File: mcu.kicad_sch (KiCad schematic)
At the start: 47 parts, among them J1 USB_C_Receptacle_USB2.0_16P, J4 Conn_01x03_Pin, J5 Conn_01x03_Pin, J6 Conn_02x04_Odd_Even, J7 AudioJack2_Ground_Switch, SW4 RotaryEncoder_Switch, SW5 RESET, SW6 BOOTSEL, U1 RP2040, U5 W25Q64JVSSIQ, U6 ADS1015IDGS, Y1 XYDBPCNANF-12MHZ

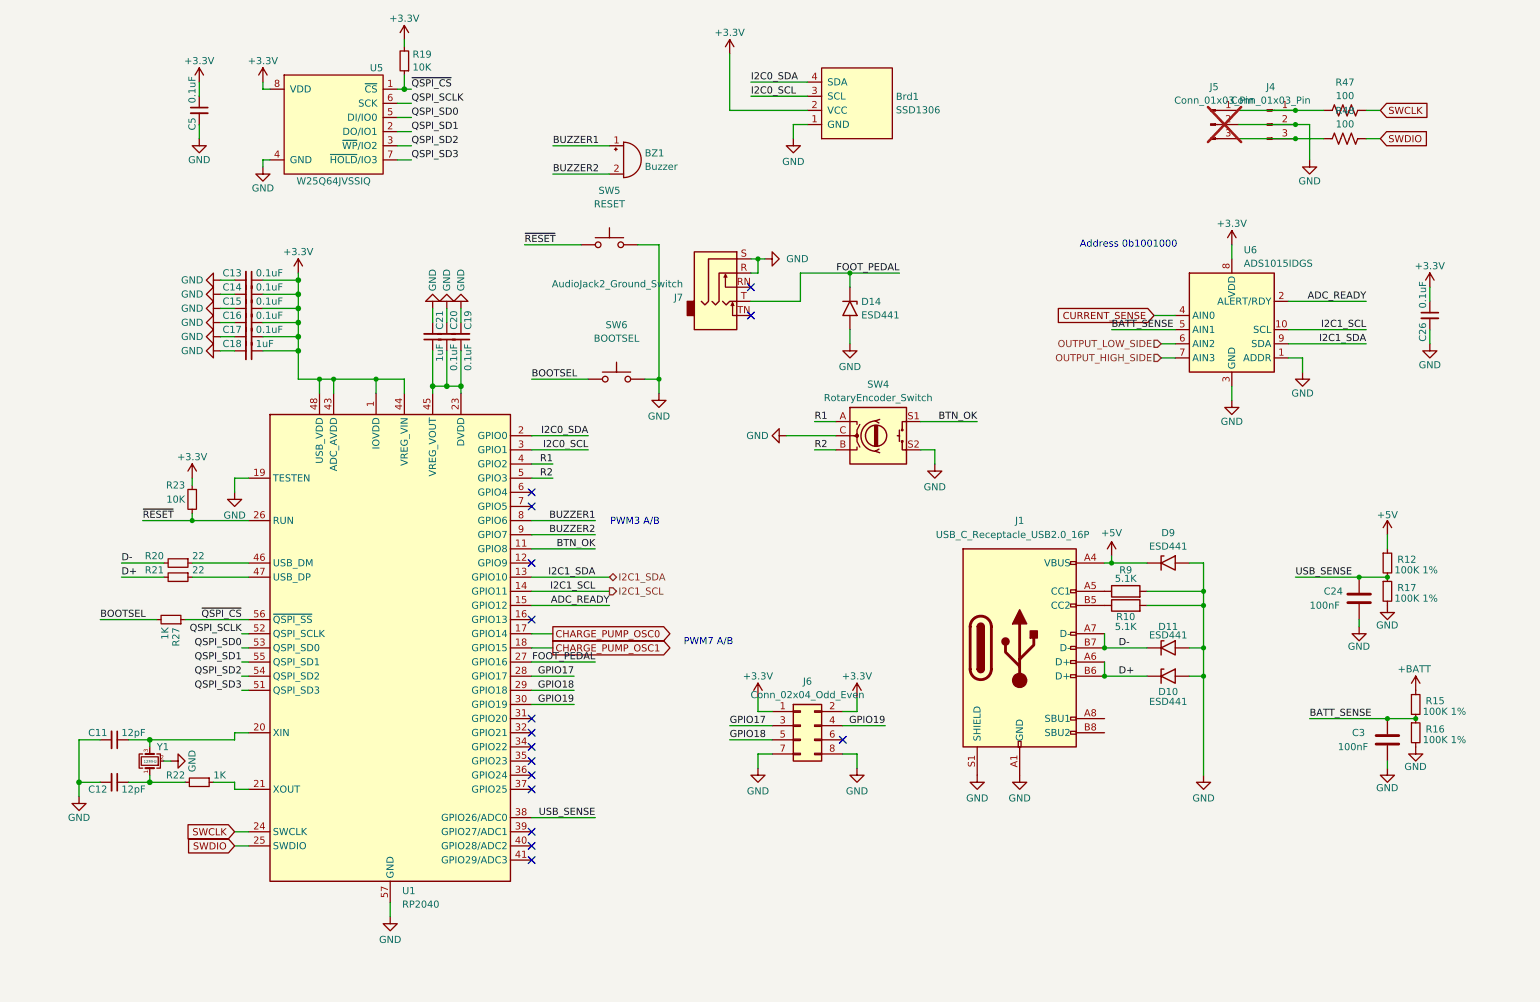
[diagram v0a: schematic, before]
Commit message: stm32g0
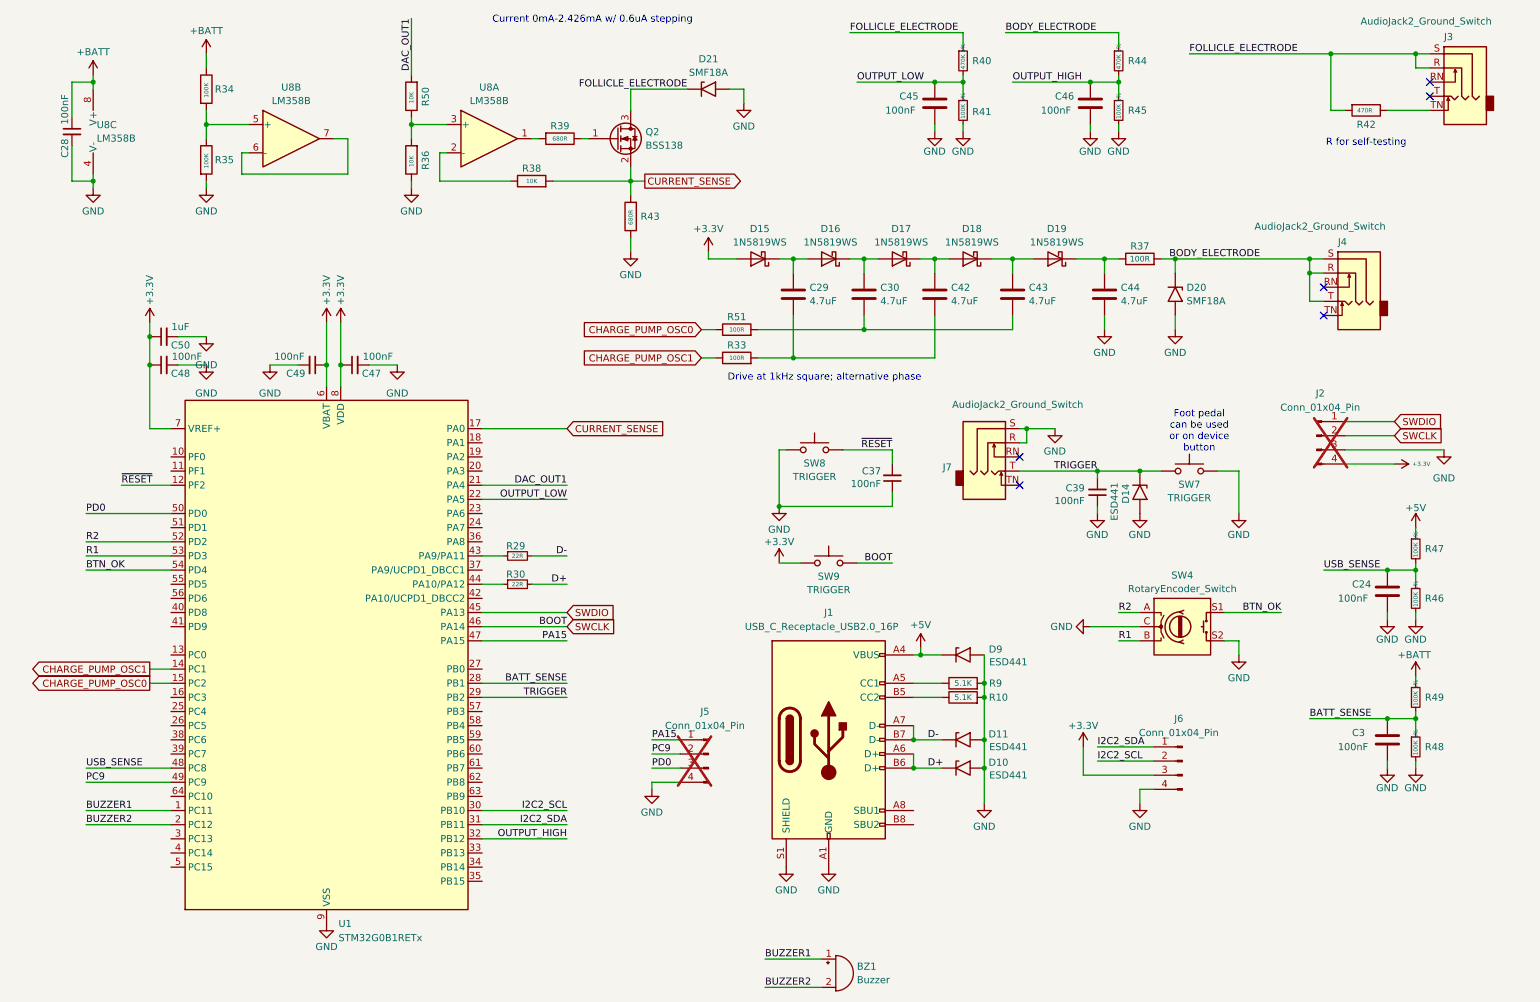
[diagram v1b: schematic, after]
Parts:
- removed Brd1: SSD1306, SSD1306:128x64OLED, symbol SSD1306-128x64_OLED:SSD1306
- removed C11, C12: 12pF, Capacitor_SMD:C_0603_1608Metric, symbol Device:C_Small
- removed C13, C14, C15, C16, C17, C19, C20, C26, C5: 0.1uF, Capacitor_SMD:C_0603_1608Metric, symbol Device:C_Small
- removed C18, C21: 1uF, Capacitor_SMD:C_0603_1608Metric, symbol Device:C_Small
- removed J4: Conn_01x03_Pin, Connector_JST:JST_SH_SM03B-SRSS-TB_1x03-1MP_P1.00mm_Horizontal, symbol Connector:Conn_01x03_Pin
- removed J5: Conn_01x03_Pin, Connector_PinHeader_2.54mm:PinHeader_1x03_P2.54mm_Vertical, symbol Connector:Conn_01x03_Pin
- removed J6: Conn_02x04_Odd_Even, Connector_PinHeader_2.54mm:PinHeader_2x04_P2.54mm_Vertical, symbol Connector_Generic:Conn_02x04_Odd_Even
- removed R12, R15, R16, R17: 100K 1%, Resistor_SMD:R_0603_1608Metric, symbol Device:R_Small
- removed R19, R23: 10K, Resistor_SMD:R_0603_1608Metric, symbol Device:R_Small
- removed R20, R21: 22, Resistor_SMD:R_0603_1608Metric, symbol Device:R_Small
- removed R22, R27: 1K, Resistor_SMD:R_0603_1608Metric, symbol Device:R_Small
- removed R47, R48: 100, Resistor_SMD:R_0603_1608Metric, symbol Device:R_US
- removed SW5: RESET, Button_Switch_SMD:SW_Push_1P1T_NO_E-Switch_TL3301NxxxxxG, symbol Switch:SW_Push
- removed SW6: BOOTSEL, Button_Switch_SMD:SW_Push_1P1T_NO_E-Switch_TL3301NxxxxxG, symbol Switch:SW_Push
- removed U1: RP2040, Package_DFN_QFN:QFN-56-1EP_7x7mm_P0.4mm_EP3.2x3.2mm, symbol MCU_RaspberryPi:RP2040
- removed U5: W25Q64JVSSIQ, Package_SO:SOIC-8_5.3x5.3mm_P1.27mm, symbol Memory_Flash_Extra:GD25Q32C
- removed U6: ADS1015IDGS, Package_SO:TSSOP-10_3x3mm_P0.5mm, symbol Analog_ADC:ADS1015IDGS
- removed Y1: XYDBPCNANF-12MHZ, Crystal:Crystal_SMD_3225-4Pin_3.2x2.5mm, symbol Device:Crystal_GND24_Small
- added C28, C37, C39, C47, C48, C49: 100nF, Capacitor_SMD:C_0603_1608Metric, symbol Device:C_Small
- added C29, C30, C42, C43, C44: 4.7uF, Capacitor_SMD:C_0603_1608Metric_Pad1.08x0.95mm_HandSolder, symbol Device:C
- added C45, C46: 100nF, Capacitor_SMD:C_0603_1608Metric, symbol Device:C
- added C50: 1uF, Capacitor_SMD:C_0603_1608Metric, symbol Device:C_Small
- added D15, D16, D17, D18, D19: 1N5819WS, Diode_SMD:D_SOD-323, symbol Diode:1N5819WS
- added D20, D21: SMF18A, Diode_SMD:D_SMF, symbol Diode:SMF18A
- added J2: Conn_01x04_Pin, Connector_PinSocket_2.54mm:PinSocket_1x04_P2.54mm_Vertical, symbol Connector:Conn_01x04_Pin
- added J3: AudioJack2_Ground_Switch, Connector_Audio:Jack_3.5mm_CUI_SJ1-3525N_Horizontal, symbol Connector_Audio:AudioJack3_SwitchTR
- added J4: AudioJack2_Ground_Switch, 2.5mm:Jack_2.5mm_PJ242_6P_12x6.2x4mm_Horizontal, symbol Connector_Audio:AudioJack3_SwitchTR
- added J5, J6: Conn_01x04_Pin, Connector_PinHeader_2.54mm:PinHeader_1x04_P2.54mm_Vertical, symbol Connector:Conn_01x04_Pin
- added Q2: BSS138, Package_TO_SOT_SMD:SOT-23, symbol Transistor_FET:BSS138
- added R29, R30: 22R, Resistor_SMD:R_0603_1608Metric, symbol Device:R_Small
- added R33, R37, R51: 100R, Resistor_SMD:R_0603_1608Metric, symbol Device:R
- added R34, R35: 100K, Resistor_SMD:R_0603_1608Metric_Pad0.98x0.95mm_HandSolder, symbol Device:R
- added R36, R38, R50: 10K, Resistor_SMD:R_0603_1608Metric_Pad0.98x0.95mm_HandSolder, symbol Device:R
- added R39, R43: 680R, Resistor_SMD:R_0603_1608Metric_Pad0.98x0.95mm_HandSolder, symbol Device:R
- added R40, R44: 470K 1%, Resistor_SMD:R_0603_1608Metric, symbol Device:R_Small
- added R41, R45, R46, R47, R48, R49: 100K 1%, Resistor_SMD:R_0603_1608Metric, symbol Device:R_Small
- added R42: 470R, Resistor_SMD:R_0603_1608Metric_Pad0.98x0.95mm_HandSolder, symbol Device:R
- added SW7, SW8, SW9: TRIGGER, Button_Switch_SMD:YZA-032-5.0W, symbol Switch:SW_Push
- added U1: STM32G0B1RETx, Package_QFP:LQFP-64_10x10mm_P0.5mm, symbol MCU_ST_STM32G0:STM32G0B1RETx
- added U8: LM358B, Package_SO:SOIC-8_3.9x4.9mm_P1.27mm, symbol Amplifier_Operational:LM358
- D10, D11, D14, D9: footprint Diode_SMD:D_0201_0603Metric -> Diode_SMD:D_0402_1005Metric; LCSC C52994072 -> C316049
- R10, R9: LCSC (none) -> C23186
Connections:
- net +3.3V: now also C47.1, C48.1, C49.1, C50.1, D15.2 (A), J2.4 (Pin_4), J6.3 (Pin_3), SW9.2, U1.6 (VBAT), U1.7 (VREF+), U1.8 (VDD)
- net +5V: now also R47.1
- net +BATT: now also C28.1, R34.1, R49.1, U8.8 (V+)
- net BATT_SENSE: now also R48.1, R49.2, U1.28 (PB1)
- net BTN_OK: now also U1.54 (PD4)
- net BUZZER1: now also U1.1 (PC11)
- net BUZZER2: now also U1.2 (PC12)
- net CHARGE_PUMP_OSC0: now also R51.1, U1.15 (PC2)
- net CHARGE_PUMP_OSC1: now also R33.1, U1.14 (PC1)
- net CURRENT_SENSE: now also Q2.2 (S), R38.2, R43.2, U1.17 (PA0)
- net D+: now also R30.2
- net D-: now also R29.2
- net GND: now also C28.2, C37.1, C39.1, C44.2, C45.2, C46.2, C47.2, C48.2, C49.2, C50.2, D20.2 (A2), D21.2 (A2), J2.3 (Pin_3), J5.4 (Pin_4), J6.4 (Pin_4), R35.2, R36.1, R41.2, R43.1, R45.2, R46.2, R48.2, SW7.1, SW8.2, U1.9 (VSS), U8.4 (V-)
- net R1: now also SW4.B, U1.53 (PD3); no longer SW4.A
- net R2: now also SW4.A, U1.52 (PD2); no longer SW4.B
- net SWCLK: now also J2.2 (Pin_2), SW9.1, U1.46 (PA14)
- net SWDIO: now also J2.1 (Pin_1), U1.45 (PA13)
- net USB_SENSE: now also R46.1, R47.2, U1.48 (PC8)
- net ~{RESET}: now also C37.2, SW8.1, U1.12 (PF2)
- net FOOT_PEDAL renamed TRIGGER
- net TRIGGER: now also C39.2, SW7.2, U1.29 (PB2)
- new net: R36.2, R50.1, U8.3 (+)
- new net: Q2.1 (G), R39.1
- new net: C43.1, D18.1 (K), D19.2 (A)
- new net: C30.2, C43.2, R51.2
- new net: R34.2, R35.1, U8.5 (+)
- new net: C44.1, D19.1 (K), R37.1
- new net: C29.1, D15.1 (K), D16.2 (A)
- new net: C29.2, C42.2, R33.2
- new net: R38.1, U8.2 (-)
- new net: C30.1, D16.1 (K), D17.2 (A)
- new net: C42.1, D17.1 (K), D18.2 (A)
- new net: R29.1, U1.43 (PA9/PA11)
- new net: R30.1, U1.44 (PA10/PA12)
- new net: R39.2, U8.1
- new net: U8.6 (-), U8.7
- new net: J3.TN, R42.1
- new net BODY_ELECTRODE: D20.1 (A1), J4.R, J4.S, J4.T, R37.2, R44.1
- new net DAC_OUT1: R50.2, U1.21 (PA4)
- new net FOLLICLE_ELECTRODE: D21.1 (A1), J3.R, J3.S, Q2.3 (D), R40.1, R42.2
- new net I2C2_SCL: J6.2 (Pin_2), U1.30 (PB10)
- new net I2C2_SDA: J6.1 (Pin_1), U1.31 (PB11)
- new net OUTPUT_HIGH: C46.1, R44.2, R45.1, U1.32 (PB12)
- new net OUTPUT_LOW: C45.1, R40.2, R41.1, U1.22 (PA5)
- new net PA15: J5.1 (Pin_1), U1.47 (PA15)
- new net PC9: J5.2 (Pin_2), U1.49 (PC9)
- new net PD0: J5.3 (Pin_3), U1.50 (PD0)
- no-connect marks 16 -> 6
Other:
- note added: "Current 0mA-2.426mA w/ 0.6uA stepping"
- note added: "Drive at 1kHz square; alternative phase"
- note added: "Foot pedal can be used or on device button"
- note added: "R for self-testing"
- note removed: "12MHz"
- note removed: "Address 0b1001000"
- note removed: "PWM3 A/B"
- note removed: "PWM7 A/B"
- moved on the sheet: BZ1, C24, D10, D11, D14, D9, J1, J7, R10, R9, SW4
